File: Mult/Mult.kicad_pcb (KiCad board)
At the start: 2 copper layers, 70.8 x 104.5 mm, 49 parts, among them J1 Conn_02x05_Odd_Even, J10 AudioJack2_SwitchT, J11 AudioJack2_SwitchT, J12 AudioJack2_SwitchT, J13 AudioJack2_SwitchT, J14 AudioJack2_SwitchT, J15 AudioJack2_SwitchT, J2 AudioJack2_SwitchT, J3 AudioJack2_SwitchT, J4 AudioJack2_SwitchT, J5 AudioJack2_SwitchT, J6 AudioJack2_SwitchT, J7 AudioJack2_SwitchT, J8 AudioJack2_SwitchT, J9 AudioJack2_SwitchT, U1 TL072, U2 TL072, U3 TL072, U4 TL072, U5 TL072, U6 TL072

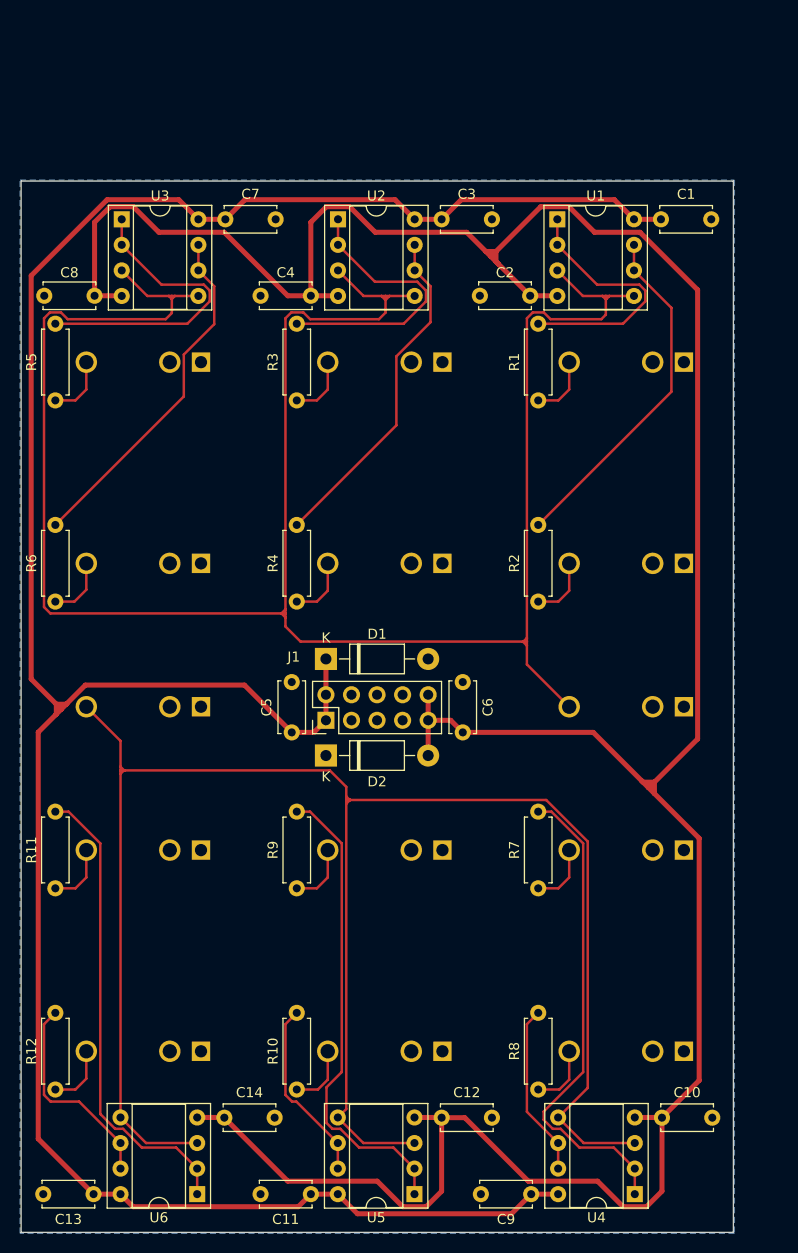
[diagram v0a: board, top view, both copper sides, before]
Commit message: Finish main set of revisions
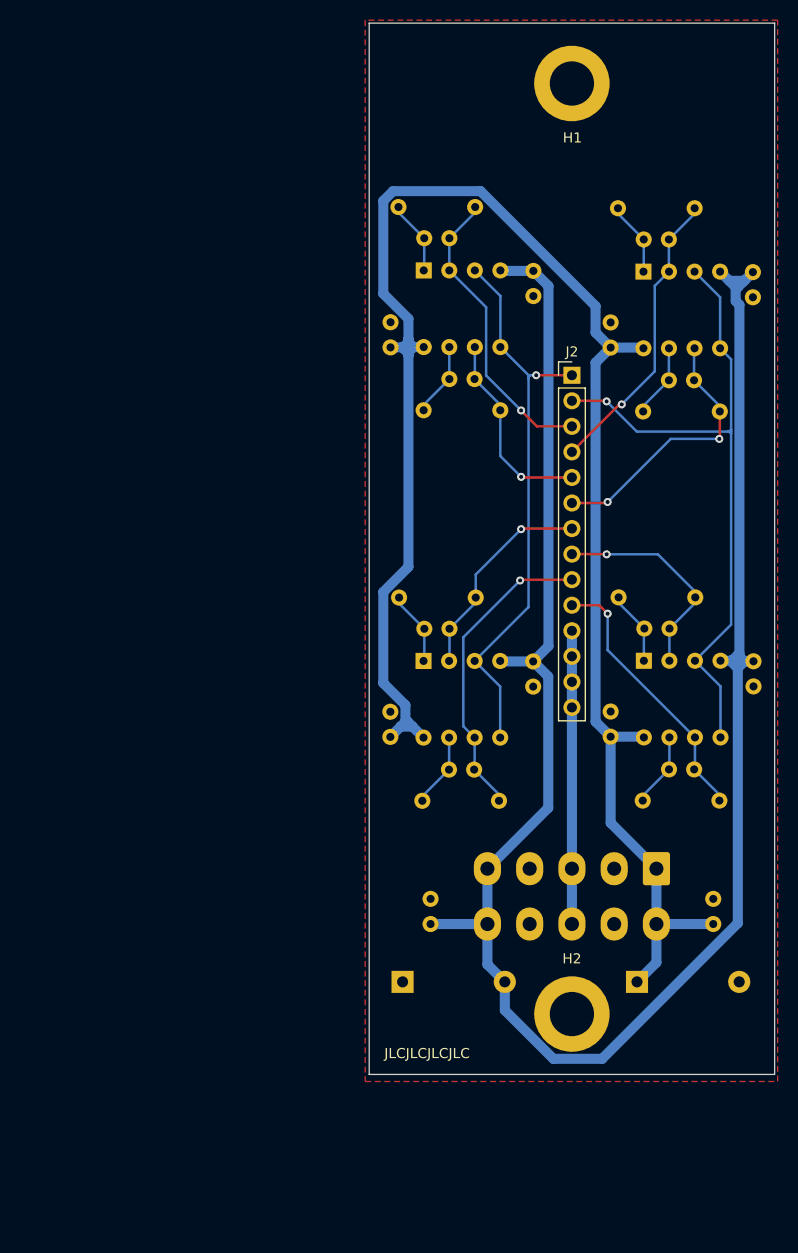
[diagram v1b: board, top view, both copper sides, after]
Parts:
- removed J10, J11, J12, J13, J14, J15, J3, J4, J5, J6, J7, J8, J9: AudioJack2_SwitchT, Connector_Audio:Jack_3.5mm_QingPu_WQP-PJ398SM_Vertical_CircularHoles
- removed R10, R11, R12, R9: 1k, Resistor_THT:R_Axial_DIN0207_L6.3mm_D2.5mm_P7.62mm_Horizontal
- removed U5, U6: TL072, Package_DIP:DIP-8_W7.62mm_Socket
- added C15: 10p, 0_Capacitor_THT:C_Disc_D5.5mm_W2.5mm_P2.50mm, B.Cu at (182.7, 55.8)
- added C16: 10p, 0_Capacitor_THT:C_Disc_D5.5mm_W2.5mm_P2.50mm, B.Cu at (185.2, 69.8)
- added C17: 10p, 0_Capacitor_THT:C_Disc_D5.5mm_W2.5mm_P2.50mm, B.Cu at (182.8, 94.5)
- added C18: 10p, 0_Capacitor_THT:C_Disc_D5.5mm_W2.5mm_P2.50mm, B.Cu at (185.2, 108.5)
- added H1: MNT_STANDOFF, 0_MountingHole:MountingHole_Pitch7.5mm_Drill3.4mm, F.Cu at (173.1, 40.3)
- added H2: MNT_STANDOFF, 0_MountingHole:MountingHole_Pitch7.5mm_Drill3.4mm, F.Cu at (173.1, 132.8)
- C1, C10, C2, C3, C4, C7, C8, C9: value 10n -> 0.1u; footprint Capacitor_THT:C_Disc_D5.0mm_W2.5mm_P5.00mm -> 0_Capacitor_THT:C_Disc_D5.5mm_W2.5mm_P2.50mm; moved to B.Cu
- C11, C12, C13, C14: value 10n -> 10p; footprint Capacitor_THT:C_Disc_D5.0mm_W2.5mm_P5.00mm -> 0_Capacitor_THT:C_Disc_D5.5mm_W2.5mm_P2.50mm; moved to B.Cu
- C5, C6: value 0.1u -> 10u; footprint Capacitor_THT:C_Disc_D5.0mm_W2.5mm_P5.00mm -> 0_Capacitor_THT:C_Disc_D5.5mm_W4.0mm_P2.50mm; moved to B.Cu
- D1, D2, R1, R2, R3, R4, R5, R6, R7, R8, U1, U2, U3, U4: moved to B.Cu
- J1: value Conn_02x05_Odd_Even -> Conn_02x05_Top_Bottom; footprint Connector_PinHeader_2.54mm:PinHeader_2x05_P2.54mm_Vertical -> Connector_Molex:Molex_Mini-Fit_Jr_5566-10A_2x05_P4.20mm_Vertical; moved to B.Cu
- J2: value AudioJack2_SwitchT -> Conn_01x14_Pin; footprint Connector_Audio:Jack_3.5mm_QingPu_WQP-PJ398SM_Vertical_CircularHoles -> Connector_PinHeader_2.54mm:PinHeader_1x14_P2.54mm_Vertical; moved to F.Cu
- moved C11 96.0 mm to (160.9, 55.7)
- moved C12 73.5 mm to (163.4, 69.7), turned to 180 degrees
- moved R6 68.7 mm to (187.8, 72.9), turned to 180 degrees
- moved C13 66.4 mm to (160.9, 94.5)
- moved R5 66.4 mm to (185.2, 52.7), turned to 180 degrees
- moved C8 65.5 mm to (191.0, 59.0), turned to -90 degrees
- moved U4 53.0 mm to (180.2, 97.7), turned to -90 degrees
- moved U3 52.1 mm to (180.2, 59.0), turned to -90 degrees
- moved C3 51.7 mm to (155.0, 105.2), turned to 90 degrees
- moved C10 46.3 mm to (191.1, 97.7), turned to -90 degrees
- moved C9 46.2 mm to (176.9, 105.2), turned to 90 degrees
- moved C5 46.0 mm to (187.1, 123.8)
- moved U2 44.7 mm to (158.3, 97.7), turned to -90 degrees
- moved D1 44.6 mm to (179.5, 129.6)
- moved C14 42.6 mm to (163.3, 108.5), turned to 180 degrees
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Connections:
- C11 pad 1: +12V -> /OUT_1_1
- C11 pad 2: GND -> Net-(C11-Pad2)
- C12 pad 1: -12V -> /OUT_1_2
- C12 pad 2: GND -> Net-(C12-Pad2)
- C13 pad 1: +12V -> /OUT_1_3
- C13 pad 2: GND -> Net-(C13-Pad2)
- C14 pad 1: -12V -> /OUT_1_4
- C14 pad 2: GND -> Net-(C14-Pad2)
- J1 pad 2: +12V -> GND
- J1 pad 3: GND -> Chassis
- J1 pad 5: GND -> -12V
- J1 pad 6: GND -> +12V
- J1 pad 8: GND -> Chassis
- J1 pad 9: -12V -> GND
- R1 pad 1: Net-(J3-PadT) -> /OUT_1_1
- R1 pad 2: Net-(R1-Pad2) -> Net-(C11-Pad2)
- R2 pad 1: Net-(J4-PadT) -> /OUT_1_2
- R2 pad 2: Net-(R2-Pad2) -> Net-(C12-Pad2)
- R3 pad 1: Net-(J5-PadT) -> /OUT_1_3
- R3 pad 2: Net-(R3-Pad2) -> Net-(C13-Pad2)
- R4 pad 1: Net-(J6-PadT) -> /OUT_1_4
- R4 pad 2: Net-(R4-Pad2) -> Net-(C14-Pad2)
- R5 pad 1: Net-(J7-PadT) -> /OUT_2_1
- R5 pad 2: Net-(R5-Pad2) -> Net-(C15-Pad2)
- R6 pad 1: Net-(J8-PadT) -> /OUT_2_2
- R6 pad 2: Net-(R6-Pad2) -> Net-(C16-Pad2)
- R7 pad 1: Net-(J10-PadT) -> /OUT_2_3
- R7 pad 2: Net-(R7-Pad2) -> Net-(C17-Pad2)
- R8 pad 1: Net-(J11-PadT) -> /OUT_2_4
- R8 pad 2: Net-(R8-Pad2) -> Net-(C18-Pad2)
- U1 pad 1: Net-(R1-Pad2) -> Net-(C11-Pad2)
- U1 pad 2: Net-(R1-Pad2) -> /OUT_1_1
- U1 pad 3: Net-(J2-PadT) -> /IN_1
- U1 pad 5: Net-(J2-PadT) -> /IN_1
- U1 pad 6: Net-(R2-Pad2) -> /OUT_1_2
- U1 pad 7: Net-(R2-Pad2) -> Net-(C12-Pad2)
- U2 pad 1: Net-(R3-Pad2) -> Net-(C13-Pad2)
- U2 pad 2: Net-(R3-Pad2) -> /OUT_1_3
- U2 pad 3: Net-(J2-PadT) -> /IN_1
- U2 pad 5: Net-(J2-PadT) -> /IN_1
- U2 pad 6: Net-(R4-Pad2) -> /OUT_1_4
- U2 pad 7: Net-(R4-Pad2) -> Net-(C14-Pad2)
- U3 pad 1: Net-(R5-Pad2) -> Net-(C15-Pad2)
- U3 pad 2: Net-(R5-Pad2) -> /OUT_2_1
- U3 pad 3: Net-(J2-PadT) -> /IN_2
- U3 pad 5: Net-(J2-PadT) -> /IN_2
- U3 pad 6: Net-(R6-Pad2) -> /OUT_2_2
- U3 pad 7: Net-(R6-Pad2) -> Net-(C16-Pad2)
- U4 pad 1: Net-(R7-Pad2) -> Net-(C17-Pad2)
- U4 pad 2: Net-(R7-Pad2) -> /OUT_2_3
- U4 pad 3: Net-(J9-PadT) -> /IN_2
- U4 pad 5: Net-(J9-PadT) -> /IN_2
- U4 pad 6: Net-(R8-Pad2) -> /OUT_2_4
- U4 pad 7: Net-(R8-Pad2) -> Net-(C18-Pad2)
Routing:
- net Net-(J2-PadT): track 217.7 -> 0.00 mm
- net Net-(J9-PadT): track 181.1 -> 0.00 mm
- net -12V: track 299.0 -> 198.3 mm
- net +12V: track 252.3 -> 177.9 mm
- net /IN_2: track 0.00 -> 68.1 mm, vias 0 -> 1
- net /IN_1: track 0.00 -> 56.6 mm, vias 0 -> 1
- net Net-(R7-Pad2): track 48.5 -> 0.00 mm
- net Net-(R9-Pad2): track 47.4 -> 0.00 mm
- net Net-(R11-Pad2): track 47.1 -> 0.00 mm
- net Net-(R6-Pad2): track 35.0 -> 0.00 mm
- net Net-(R2-Pad2): track 34.9 -> 0.00 mm
- net Net-(R4-Pad2): track 34.0 -> 0.00 mm
- net /OUT_1_4: track 0.00 -> 30.9 mm, vias 0 -> 1
- net Net-(R5-Pad2): track 30.5 -> 0.00 mm
- net /OUT_1_1: track 0.00 -> 29.9 mm, vias 0 -> 1
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- added copper zone on F.Cu, net GND
- removed copper zone on B.Cu, net GND
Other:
- board size 70.8 x 104.5 mm -> 40.3 x 104.5 mm
- board text added: "JLCJLCJLCJLC"
- board text added: "Mult V1 Matthew Taylor"
